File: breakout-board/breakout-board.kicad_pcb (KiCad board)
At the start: 2 copper layers, 91.4 x 91.4 mm, 9 parts, among them J1 Screw_Terminal_1x08, P0 CONN_02X25, P1 CONN_02X25

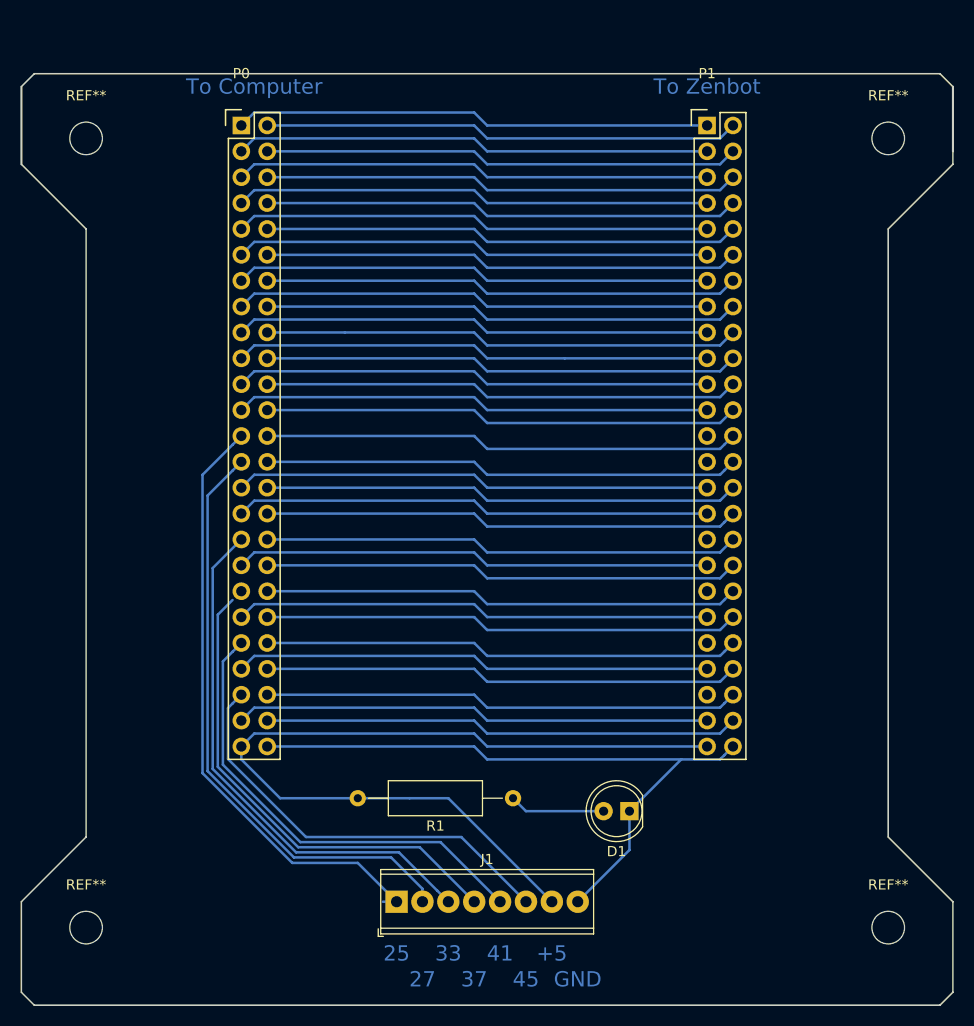
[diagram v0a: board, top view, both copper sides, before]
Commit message: breakout-board: next prototype is ready
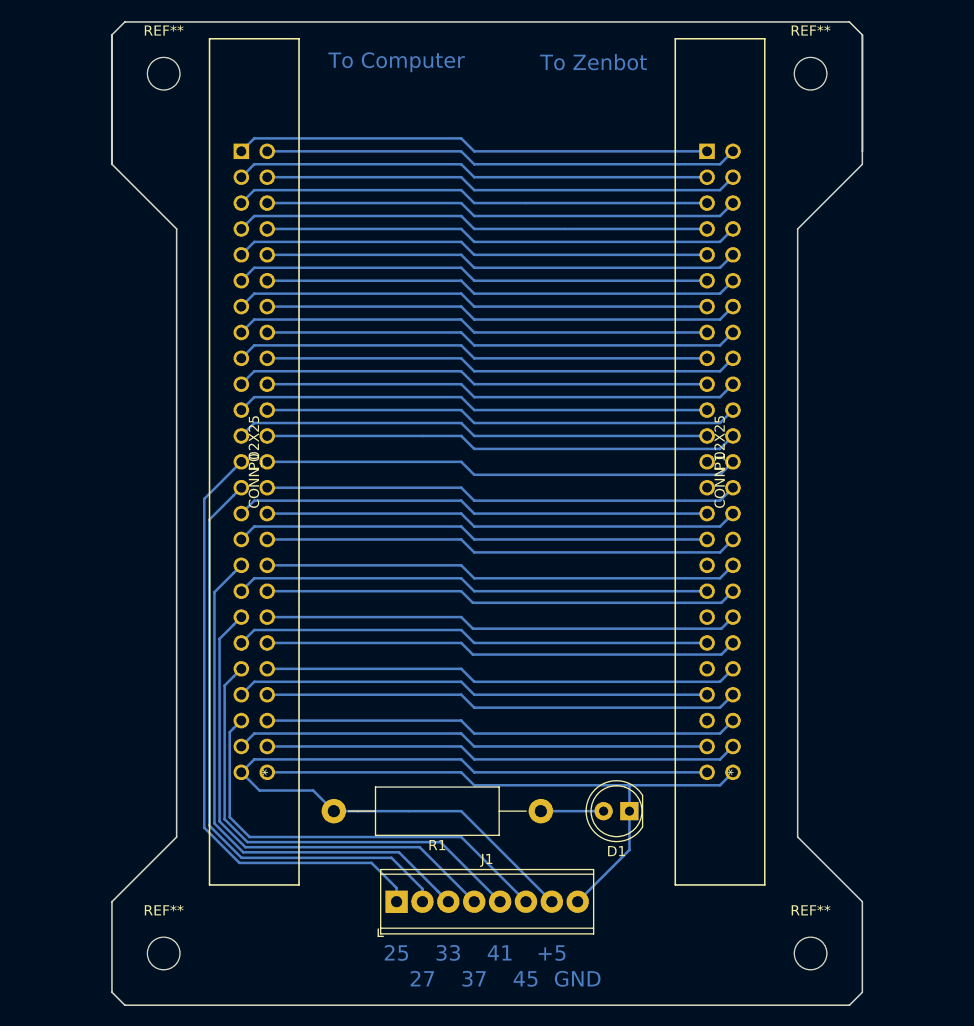
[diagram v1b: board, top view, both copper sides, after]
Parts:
- removed the REF** at (174.0, 44.5)
- removed the REF** at (95.2, 121.9)
- removed the REF** at (95.2, 44.5)
- removed the REF** at (174.0, 121.9)
- added REF**: MountingHole_3.2mm_M3, MountingHole:MountingHole_3.2mm_M3, F.Cu at (102.9, 38.1)
- added REF**: MountingHole_3.2mm_M3, MountingHole:MountingHole_3.2mm_M3, F.Cu at (166.4, 38.1)
- added REF**: MountingHole_3.2mm_M3, MountingHole:MountingHole_3.2mm_M3, F.Cu at (166.4, 124.5)
- added REF**: MountingHole_3.2mm_M3, MountingHole:MountingHole_3.2mm_M3, F.Cu at (102.9, 124.5)
- P0, P1: footprint Pin_Headers:Pin_Header_Straight_2x25 -> zenbot:TE-Connectivity_1-5499923-0
- R1: footprint Resistor_THT:R_Axial_DIN0309_L9.0mm_D3.2mm_P15.24mm_Horizontal -> Resistor_THT:R_Axial_DIN0414_L11.9mm_D4.5mm_P20.32mm_Horizontal
- moved P0 63.6 mm to (113.0, 106.7), turned to 270 degrees
- moved P1 63.6 mm to (158.8, 106.7), turned to 270 degrees
- moved R1 3.01 mm to (139.9, 110.5)
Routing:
- net Net-(D1-Pad1): track 65.0 -> 60.3 mm
- net Net-(D1-Pad2): track 9.42 -> 6.16 mm
- net Net-(J1-Pad3): track 52.2 -> 54.1 mm
- net Net-(J1-Pad7): track 84.3 -> 82.5 mm
- net Net-(J1-Pad4): track 47.6 -> 49.2 mm
- net Net-(J1-Pad6): track 41.9 -> 42.5 mm
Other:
- board size 91.4 x 91.4 mm -> 73.7 x 96.5 mm
